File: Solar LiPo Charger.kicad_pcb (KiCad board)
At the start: 2 copper layers, 50.2 x 34.3 mm, 37 parts, among them J1 Barrel_Jack, Q1 DMN3404L-7, U1 bq24650

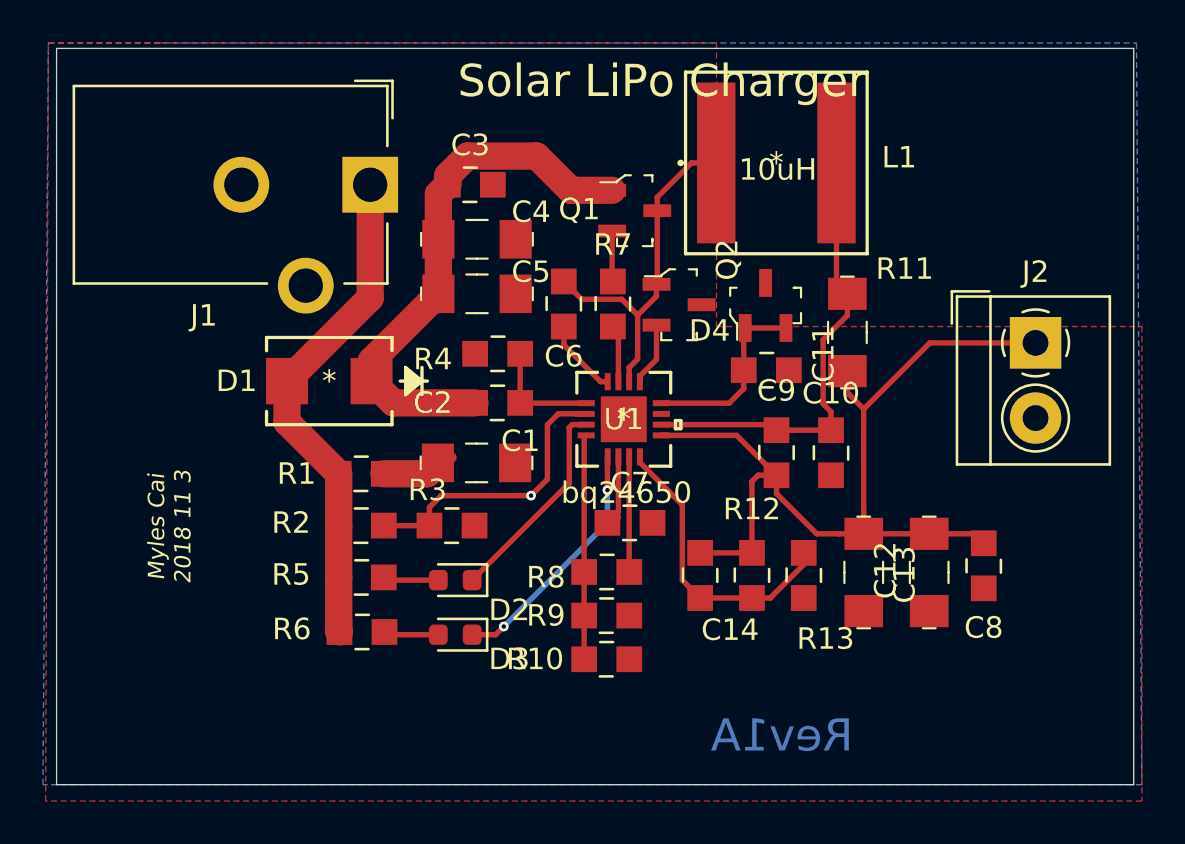
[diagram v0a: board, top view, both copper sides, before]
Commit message: Rev2B Final
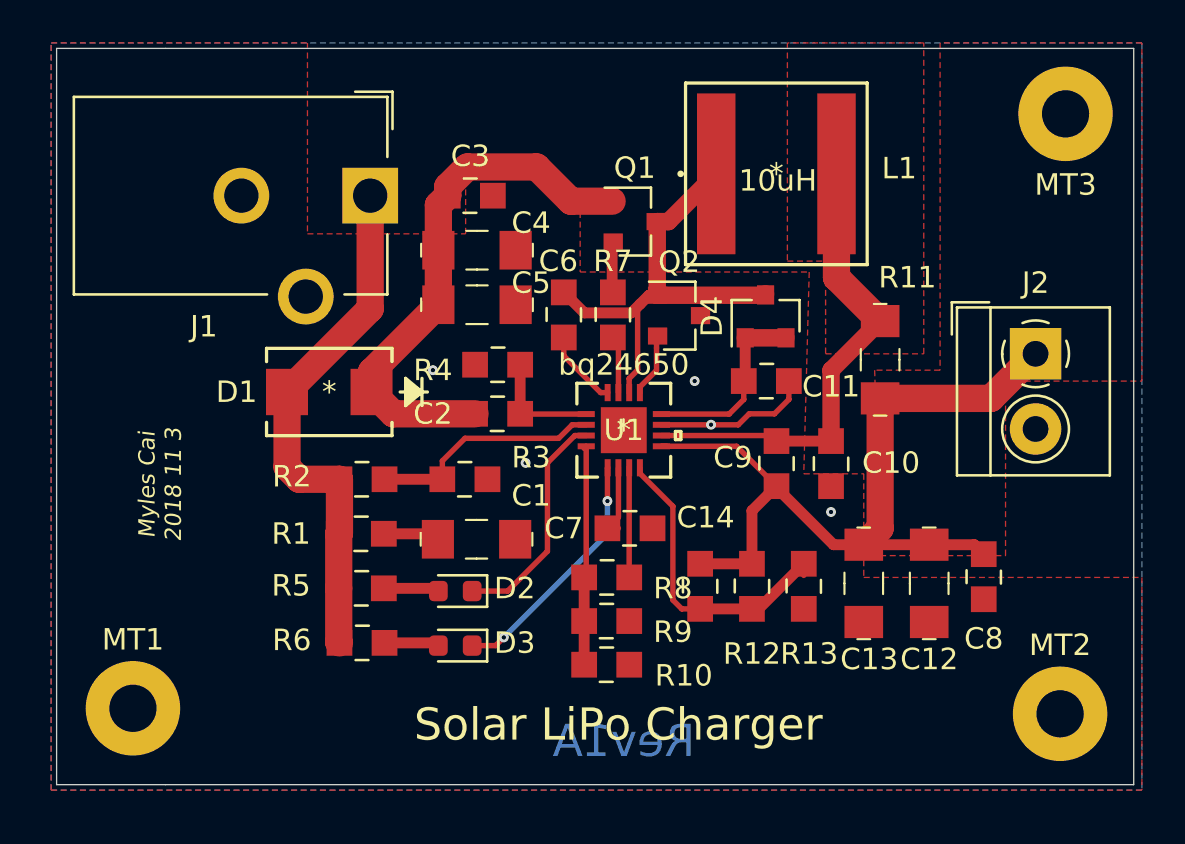
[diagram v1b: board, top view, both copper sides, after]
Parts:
- added MT1: MountingHole_2.2mm_M2_Pad, MountingHole:MountingHole_2.2mm_M2_Pad, F.Cu at (107.7, 98.0)
- added MT2: MountingHole_2.2mm_M2_Pad, MountingHole:MountingHole_2.2mm_M2_Pad, F.Cu at (150.9, 98.3)
- added MT3: MountingHole_2.2mm_M2_Pad, MountingHole:MountingHole_2.2mm_M2_Pad, F.Cu at (151.1, 70.4)
- D4: footprint digikey-footprints:SOT-23-3-MC2 -> Diode_SMD:D_SOT-23_ANK-MC
- Q1, Q2: footprint digikey-footprints:SOT-23-3 -> Diode_SMD:D_SOT-23-Q
- moved C1 3.56 mm to (123.7, 90.2)
- moved R1 2.79 mm to (118.3, 89.9)
- moved R3 2.24 mm to (123.2, 87.4)
- moved R2 2.16 mm to (118.4, 87.4)
- moved R11 1.98 mm to (142.5, 81.8)
- moved C12 0.51 mm to (144.8, 92.2)
- moved C13 0.51 mm to (141.7, 92.2)
- moved C3 0.51 mm to (123.4, 74.2)
- moved C5 0.51 mm to (123.7, 79.2)
- moved D3 0.51 mm to (122.7, 95.1)
- moved D4 0.51 mm to (137.2, 79.8)
- moved J1 0.51 mm to (118.7, 74.2)
- moved J2 0.51 mm to (149.7, 81.5)
- moved R4 0.51 mm to (124.7, 84.3)
- moved R5 0.51 mm to (118.3, 92.5)
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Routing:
- net GND: track 0.00 -> 7.29 mm, vias 0 -> 5
- net BTST: track 16.6 -> 21.7 mm
- net SRN: track 42.0 -> 39.1 mm
- net MPPSET: track 13.6 -> 10.9 mm, vias 1 -> 0
- net Vsolar: track 23.4 -> 24.6 mm
- net SRP: track 21.3 -> 22.2 mm
- net Net-(D2-Pad1): track 10.0 -> 10.9 mm
- net VFB: track 13.7 -> 14.5 mm
- added copper zone on F.Cu, net SRN
- added copper zone on F.Cu, net SRP
